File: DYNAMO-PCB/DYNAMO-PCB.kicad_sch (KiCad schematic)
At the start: 21 parts, among them J17 USB3_A, J18 USB3_A, J19 USB3_A, J2 USB3_A, J20 USB3_A, J21 USB3_A, J22 USB3_A, J23 USB3_A, J24 USB3_A, J25 USB3_A, J26 USB_C_Receptacle_USB2.0_16P, J27 USB_C_Receptacle_USB2.0_16P, J28 USB_C_Receptacle_USB2.0_16P, J29 USB_C_Receptacle_USB2.0_16P, J3 Conn_01x03_Pin, J30 USB_C_Receptacle_USB2.0_16P

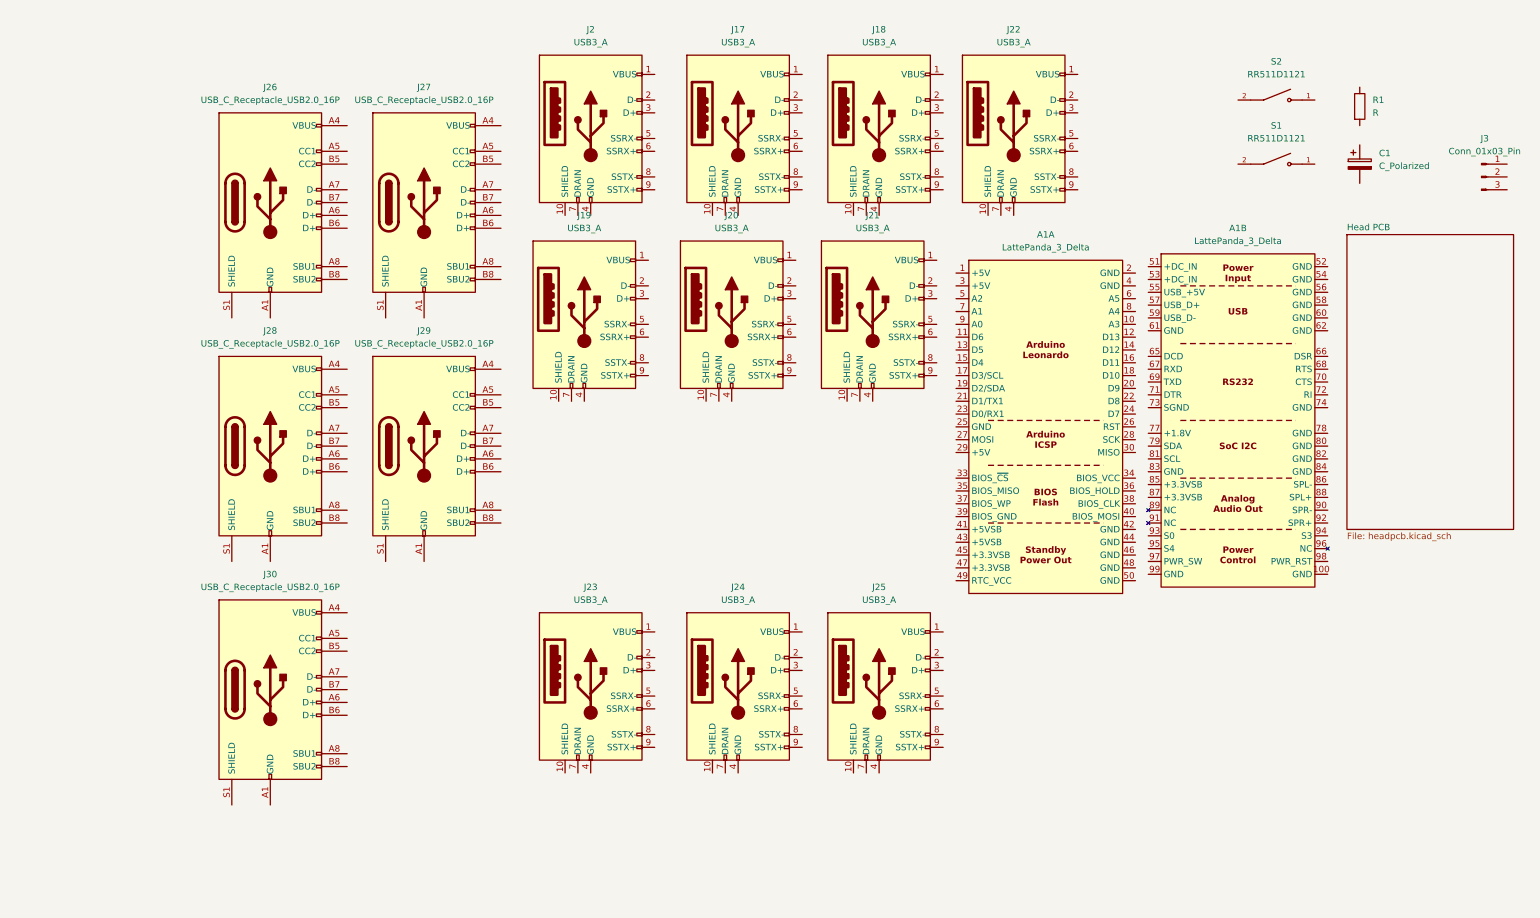
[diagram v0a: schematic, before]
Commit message: schematic wip
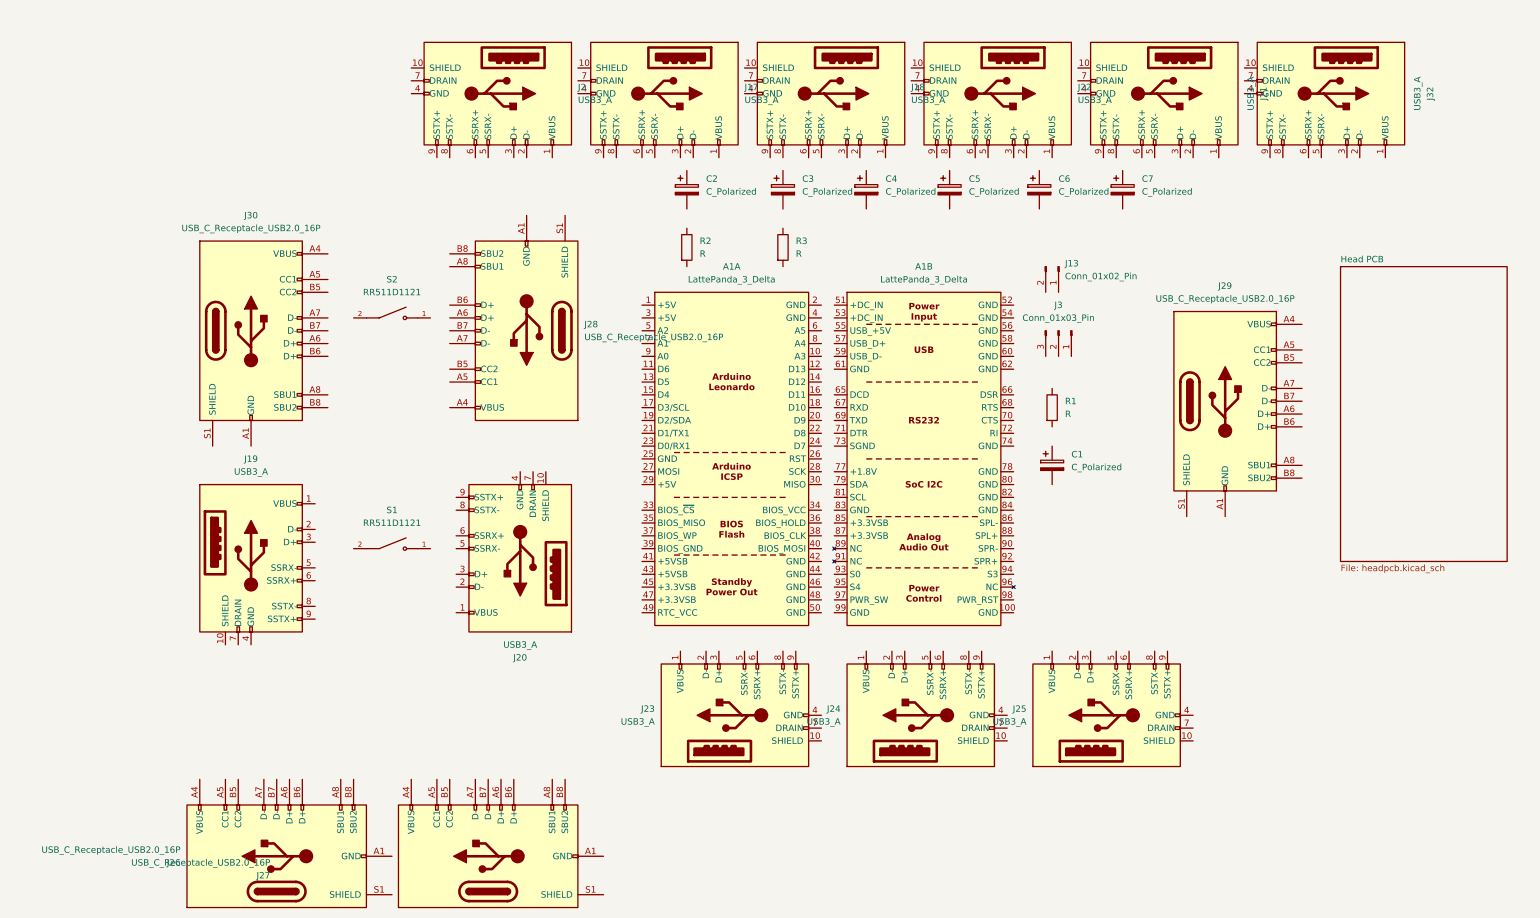
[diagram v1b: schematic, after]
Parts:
- added C2, C3, C4, C5, C6, C7: C_Polarized, Capacitor_THT:CP_Radial_D10.0mm_P5.00mm, symbol Device:C_Polarized
- added J13: Conn_01x02_Pin, Connector_PinHeader_2.54mm:PinHeader_1x02_P2.54mm_Vertical, symbol Connector:Conn_01x02_Pin
- added J32: USB3_A, 692122030100:692122030100, symbol Connector:USB3_A
- added R2, R3: R, Resistor_THT:R_Axial_DIN0309_L9.0mm_D3.2mm_P12.70mm_Horizontal, symbol Device:R
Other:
- moved on the sheet: A1A, A1B, C1, J17, J18, J19, J2, J20, J21, J22, J23, J24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

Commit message: schematic wip
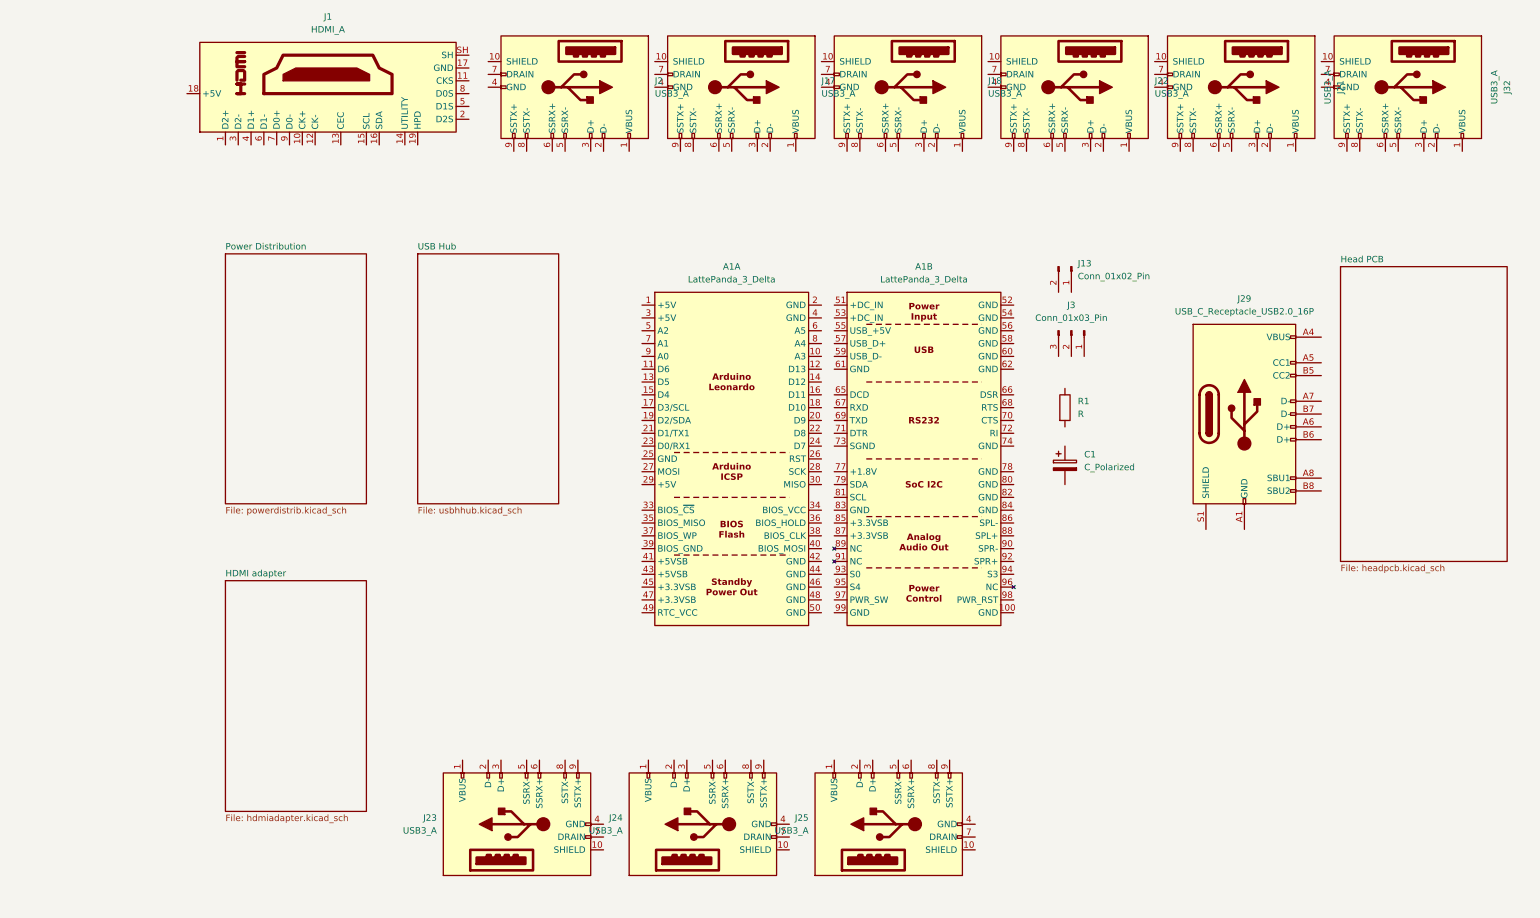
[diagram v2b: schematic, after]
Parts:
- removed C2, C3, C4, C5, C6, C7: C_Polarized, Capacitor_THT:CP_Radial_D10.0mm_P5.00mm, symbol Device:C_Polarized
- removed J19, J20: USB3_A, 692122030100:692122030100, symbol Connector:USB3_A
- removed J26, J27, J28, J30: USB_C_Receptacle_USB2.0_16P, Connector_USB:USB_C_Receptacle_GCT_USB4105-xx-A_16P_TopMnt_Horizontal, symbol Connector:USB_C_Receptacle_USB2.0_16P
- removed R2, R3: R, Resistor_THT:R_Axial_DIN0309_L9.0mm_D3.2mm_P12.70mm_Horizontal, symbol Device:R
- removed S1, S2: RR511D1121, RR511D1121:E-SWITCH_RR511D1121, symbol RR511D1121:RR511D1121
- added J1: HDMI_A, Connector_Video:HDMI_A_Molex_208658-1001_Horizontal, symbol Connector:HDMI_A
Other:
- added sheet HDMI adapter (hdmiadapter.kicad_sch)
- added sheet Power Distribution (powerdistrib.kicad_sch)
- added sheet USB Hub (usbhhub.kicad_sch)
- moved on the sheet: C1, J13, J17, J18, J2, J21, J22, J23, J24, J25, J29, J3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
